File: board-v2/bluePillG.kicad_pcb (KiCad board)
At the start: 2 copper layers, 35.6 x 50.8 mm, 34 parts, among them IC1 STM32G431C6T6, J1 Conn_02x03_Odd_Even, J2 Conn_01x20_Male, J3 Conn_01x04_Male, J4 Conn_01x20_Male, U1 LM1117-3.3, Y1 32.768kHz, Y2 8MHz

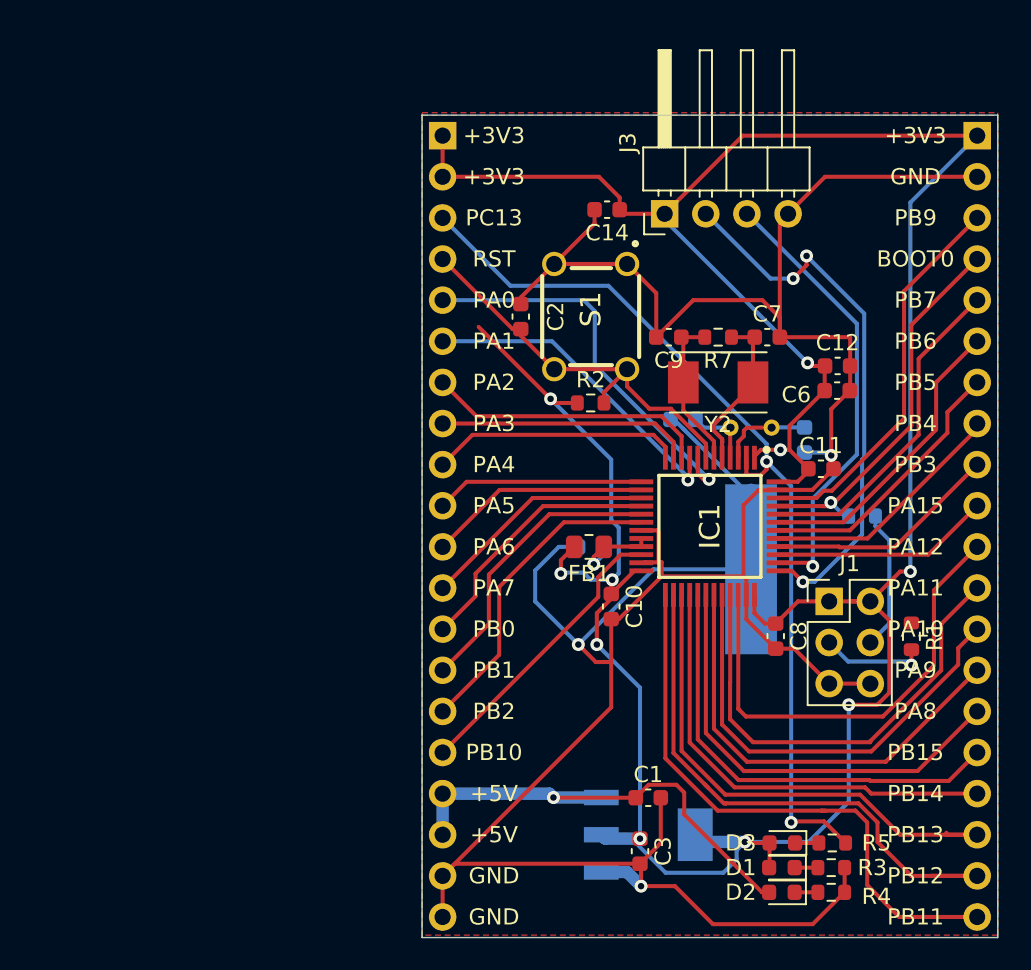
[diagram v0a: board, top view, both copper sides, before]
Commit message: board v2
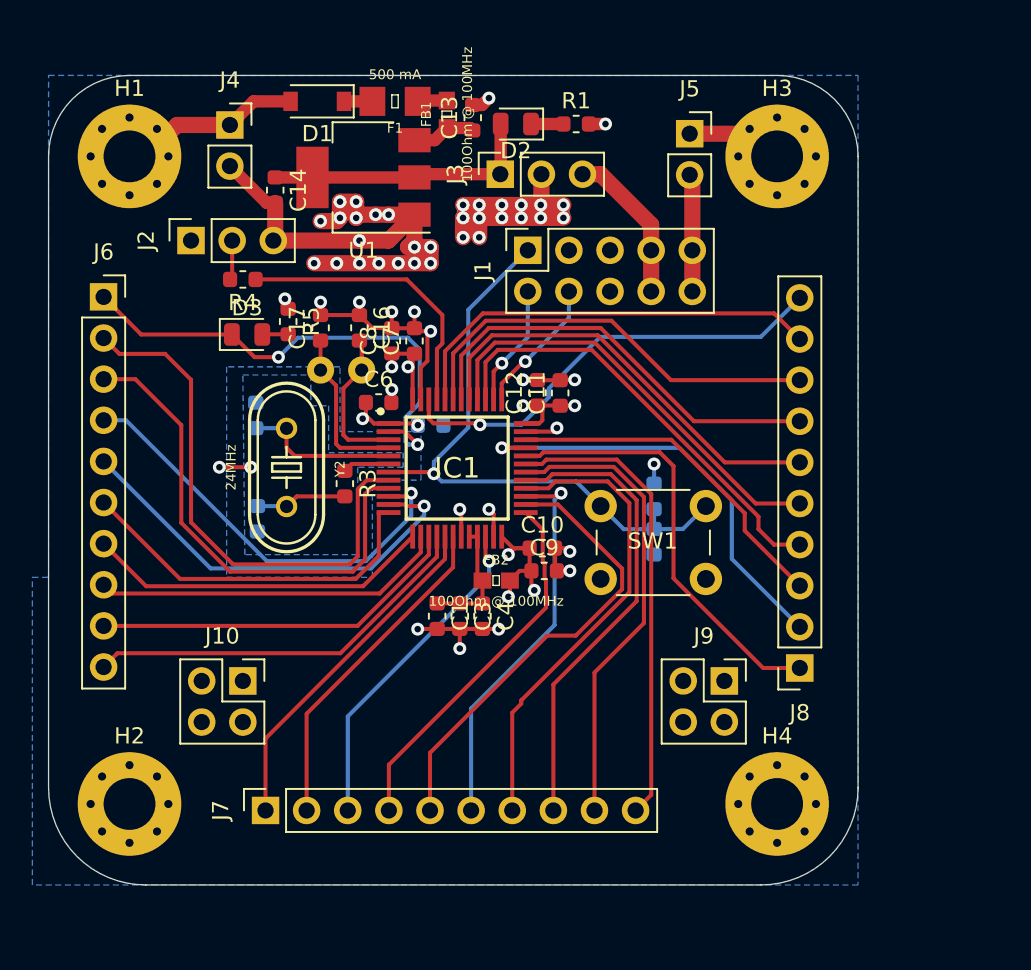
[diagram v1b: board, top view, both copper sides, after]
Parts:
- removed C2: 0.1uF, Capacitor_SMD:C_0603_1608Metric
- removed R6, R7: 100k, Resistor_SMD:R_0603_1608Metric
- removed S1: FSM4JH, FSM4JH:FSM4JH
- added C15: 100nF, Capacitor_SMD:C_0603_1608Metric, B.Cu at (66.4, 70.8)
- added C16: 6.8pF, Capacitor_SMD:C_0603_1608Metric, F.Cu at (48.2, 57.6)
- added C17: 6.8pF, Capacitor_SMD:C_0603_1608Metric, F.Cu at (45.8, 57.6)
- added C18: 20pF, Capacitor_SMD:C_0603_1608Metric, B.Cu at (41.8, 63.0)
- added C19: 20pF, Capacitor_SMD:C_0603_1608Metric, B.Cu at (41.9, 69.4)
- added F1: 500 mA, Resistors:1206, F.Cu at (50.4, 43.6)
- added FB2: 100Ohm @ 100MHz, Resistors:0603, F.Cu at (56.6, 73.2)
- added H1: MountingHole_Pad, MountingHole:MountingHole_3.2mm_M3_Pad_Via, F.Cu at (34.0, 47.0)
- added H2: MountingHole_Pad, MountingHole:MountingHole_3.2mm_M3_Pad_Via, F.Cu at (34.0, 87.0)
- added H3: MountingHole_Pad, MountingHole:MountingHole_3.2mm_M3_Pad_Via, F.Cu at (74.0, 47.0)
- added H4: MountingHole_Pad, MountingHole:MountingHole_3.2mm_M3_Pad_Via, F.Cu at (74.0, 87.0)
- added J10: Conn_02x02_Top_Bottom, Connector_PinSocket_2.54mm:PinSocket_2x02_P2.54mm_Vertical, F.Cu at (41.0, 79.4)
- added J5: Conn_01x02_Male, Connector_PinSocket_2.54mm:PinSocket_1x02_P2.54mm_Vertical, F.Cu at (68.6, 45.6)
- added J6: Conn_01x10_Male, Connector_PinSocket_2.54mm:PinSocket_1x10_P2.54mm_Vertical, F.Cu at (32.4, 55.7)
- added J7: Conn_01x10_Male, Connector_PinSocket_2.54mm:PinSocket_1x10_P2.54mm_Vertical, F.Cu at (42.4, 87.4)
- added J8: Conn_01x10_Male, Connector_PinSocket_2.54mm:PinSocket_1x10_P2.54mm_Vertical, F.Cu at (75.4, 78.6)
- added J9: Conn_02x02_Top_Bottom, Connector_PinSocket_2.54mm:PinSocket_2x02_P2.54mm_Vertical, F.Cu at (70.7, 79.4)
- added SW1: SW_Push, Button_Switch_THT:SW_PUSH_6mm_H5mm, F.Cu at (63.1, 68.6)
- C1, C3: value 0.1uF -> 1uF
- C10, C6, C8: value 0.1uF -> 100nF
- C11: value 0.1uF -> 10uF
- C12: value 10uF -> 100nF
- C13: value 0.1uF -> 10u; moved to F.Cu
- C14: value 0.1uF -> 10u
- C4: value 20p -> 100nF; moved to F.Cu
- C5, C7, C9: value 20p -> 10uF
- D1: value LED -> 1N5819; footprint LED_SMD:LED_0603_1608Metric -> Diode_SMD:D_SOD-123
- D2, D3: footprint LED_SMD:LED_0603_1608Metric -> LED_SMD:LED_0805_2012Metric
- FB1: value Ferrite_Bead -> 100Ohm @ 100MHz; footprint Resistor_SMD:R_0805_2012Metric -> Resistors:0603
- IC1: value STM32G431C6T6 -> STM32G431C6T6-STM32G431C6T6
- J1: value Conn_02x03_Odd_Even -> Conn_02x05_Odd_Even; footprint Connector_PinHeader_2.54mm:PinHeader_2x03_P2.54mm_Vertical -> Connector_PinSocket_2.54mm:PinSocket_2x05_P2.54mm_Vertical
- J2: value Conn_01x20_Male -> Conn_01x03_Male; footprint Connector_PinHeader_2.54mm:PinHeader_1x20_P2.54mm_Vertical -> Connector_PinSocket_2.54mm:PinSocket_1x03_P2.54mm_Vertical; moved to F.Cu
- J3: value Conn_01x04_Male -> Conn_01x03_Male; footprint Connector_PinHeader_2.54mm:PinHeader_1x04_P2.54mm_Horizontal -> Connector_PinSocket_2.54mm:PinSocket_1x03_P2.54mm_Vertical
- J4: value Conn_01x20_Male -> Conn_01x02_Male; footprint Connector_PinHeader_2.54mm:PinHeader_1x20_P2.54mm_Vertical -> Connector_PinSocket_2.54mm:PinSocket_1x02_P2.54mm_Vertical; moved to F.Cu
- R1: value 100k -> 2.2k
- R2: moved to B.Cu
- R3: value 1k -> 330
- R4: value 1k -> 10k
- R5: value 1k -> 2.2k
- U1: value LM1117-3.3 -> AMS1117-3.3; footprint mod:SOT-223-4 -> Package_TO_SOT_SMD:SOT-223-3_TabPin2; moved to F.Cu
- Y1: footprint Crystal:Crystal_AT310_D3.0mm_L10.0mm_Horizontal_1EP_style1 -> Clocks:CRYSTAL-PTH-2X6-CYL
- Y2: value 8MHz -> 24MHz; footprint Crystal:Crystal_SMD_Abracon_ABM7-2Pin_6.0x3.5mm -> Clocks:HC49U
- moved D1 55.4 mm to (45.6, 43.6)
- moved R4 52.5 mm to (41.0, 54.6), turned to 180 degrees
- moved D2 50.2 mm to (57.9, 45.0)
- moved R5 46.5 mm to (43.8, 57.2), turned to 270 degrees
- moved J4 46.2 mm to (40.2, 45.1), turned to 0 degrees
- moved D3 45.6 mm to (41.3, 58.0), turned to 0 degrees
- moved U1 44.2 mm to (48.5, 48.3), turned to 180 degrees
- moved R3 38.3 mm to (47.3, 67.2), turned to 270 degrees
- moved R1 37.8 mm to (61.6, 45.0), turned to 0 degrees
- moved C8 29.9 mm to (50.2, 58.4), turned to 90 degrees
- moved J1 28.6 mm to (58.6, 52.8), turned to 90 degrees
- moved C6 28.3 mm to (49.4, 62.2)
- moved FB1 28.1 mm to (53.6, 44.4), turned to 90 degrees
- moved C13 27.5 mm to (55.2, 44.6), turned to 90 degrees
- moved Y2 27.2 mm to (43.7, 66.2), turned to 270 degrees
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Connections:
- C1 pad 1: +5V -> +3.3VA
- C1 pad 2: Earth -> GND
- C10 pad 2: Earth -> GND
- C11 pad 2: Earth -> GND
- C12 pad 2: Earth -> GND
- C13 pad 1: +3.3VA -> Net-(C13-Pad1)
- C13 pad 2: Earth -> GND
- C14 pad 1: +3V3 -> +3.3VP
- C14 pad 2: Earth -> GND
- C3 pad 1: +3V3 -> +3.3VA
- C3 pad 2: Earth -> GND
- C4 pad 1: Net-(C4-Pad1) -> +3.3VA
- C4 pad 2: Earth -> GND
- C5 pad 1: Net-(C5-Pad1) -> +3V3
- C5 pad 2: Earth -> GND
- C6 pad 2: Earth -> GND
- C7 pad 1: Net-(C7-Pad1) -> +3V3
- C7 pad 2: Earth -> GND
- C8 pad 2: Earth -> GND
- C9 pad 1: Net-(C9-Pad1) -> +3V3
- C9 pad 2: Earth -> GND
- D1 pad 2: +3V3 -> VCC
- D2 pad 2: +5V -> +3.3VP
- D3 pad 1: Net-(D3-Pad1) -> PC13
- D3 pad 2: +3V3 -> Net-(D3-Pad2)
- FB1 pad 1: +3.3VA -> Net-(C13-Pad1)
- FB1 pad 2: +3V3 -> Net-(F1-Pad1)
- IC1 pad 10: /PA2 -> PA2
- IC1 pad 11: /PA3 -> PA3
- IC1 pad 12: /PA4 -> PA4
- IC1 pad 13: /PA5 -> PA5
- IC1 pad 14: /PA6 -> PA6
- IC1 pad 15: /PA7 -> PA7
- IC1 pad 16: /PB0 -> PB0
- IC1 pad 17: /PB1 -> PB1
- IC1 pad 18: /PB2 -> PB2
- IC1 pad 19: Earth -> GND
- IC1 pad 2: /PC13 -> PC13
- IC1 pad 22: /PB10 -> PB10
- IC1 pad 23: Earth -> GND
- IC1 pad 25: /PB11 -> PB11
- IC1 pad 26: /PB12 -> PB12
- IC1 pad 27: /PB13 -> PB13
- IC1 pad 28: /PB14 -> PB14
- IC1 pad 29: /PB15 -> PB15
- IC1 pad 3: Net-(C4-Pad1) -> OSC32_IN
- IC1 pad 30: /PA8 -> PA8
- IC1 pad 31: /PA9 -> PA9
- IC1 pad 32: /PA10 -> PA10
- IC1 pad 33: /PA11 -> PA11
- IC1 pad 34: /PA12 -> PA12
- IC1 pad 35: Earth -> GND
- IC1 pad 37: /SWDIO -> SWDIO
- IC1 pad 38: /SWCLK -> SWCLK
- IC1 pad 39: /PA15 -> PA15
- IC1 pad 4: Net-(C5-Pad1) -> OSC32_OUT
- IC1 pad 40: /PB3 -> PB3
- IC1 pad 41: /PB4 -> PB4
- IC1 pad 42: /PB5 -> PB5
- IC1 pad 43: /PB6 -> PB6
- IC1 pad 44: /PB7 -> PB7
- IC1 pad 45: /BOOT0 -> BOOT0
- IC1 pad 46: /PB9 -> PB9
- IC1 pad 47: Earth -> GND
- IC1 pad 5: Net-(C7-Pad1) -> OSC_IN
- IC1 pad 6: Net-(C9-Pad1) -> OSC_OUT
- IC1 pad 7: /RESET -> NRST
- IC1 pad 8: /PA0 -> PA0
- IC1 pad 9: /PA1 -> PA1
- J1 pad 1: +3V3 -> NRST
- J1 pad 2: +3V3 -> SWCLK
- J1 pad 3: Net-(J1-Pad3) -> SWIW
- J1 pad 4: Net-(J1-Pad4) -> SWDIO
- J1 pad 5: Earth -> GND
- J1 pad 6: Earth -> GND
- J2 pad 2: +3V3 -> Net-(J2-Pad2)
- J2 pad 3: /PC13 -> GND
- J3 pad 1: +3V3 -> +3.3VP
- J3 pad 2: /SWDIO -> +3V3
- J3 pad 3: /SWCLK -> +3V3S
- J4 pad 1: +3V3 -> VCC
- J4 pad 2: Earth -> GND
- R1 pad 1: /BOOT1 -> Net-(D2-Pad1)
- R1 pad 2: Net-(J1-Pad3) -> GND
- R2 pad 2: /RESET -> NRST
- R3 pad 1: Net-(D1-Pad1) -> OSC_OUT
- R3 pad 2: Earth -> Net-(C19-Pad1)
- R4 pad 1: Net-(D2-Pad1) -> BOOT0
- R4 pad 2: Earth -> Net-(J2-Pad2)
- R5 pad 1: Net-(D3-Pad1) -> +3V3
- R5 pad 2: /PC13 -> Net-(D3-Pad2)
- U1 pad 1: Earth -> GND
- U1 pad 2: +3V3 -> +3.3VP
- U1 pad 3: +5V -> Net-(C13-Pad1)
- Y1 pad 1: Net-(C4-Pad1) -> OSC32_IN
- Y1 pad 2: Net-(C5-Pad1) -> OSC32_OUT
- Y2 pad 1: Net-(C7-Pad1) -> OSC_IN
- Y2 pad 2: Net-(C9-Pad1) -> Net-(C19-Pad1)
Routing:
- net Earth: track 206.4 -> 0.00 mm, vias 3 -> 0
- net +3V3: track 196.8 -> 57.0 mm, vias 10 -> 25
- net GND: track 0.00 -> 74.2 mm, vias 0 -> 37
- net /PC13: track 56.6 -> 0.00 mm, vias 2 -> 0
- net VCC: track 0.00 -> 46.9 mm
- net NRST: track 0.00 -> 39.2 mm, vias 0 -> 1
- net /PB11: track 35.9 -> 0.00 mm
- net /PB12: track 35.5 -> 0.00 mm
- net /SWDIO: track 34.2 -> 0.00 mm, vias 3 -> 0
- net PA0: track 0.00 -> 33.1 mm
- net /PB13: track 32.1 -> 0.00 mm
- net PC13: track 0.00 -> 30.9 mm, vias 0 -> 2
- net PA1: track 0.00 -> 30.6 mm
- net +5V: track 37.2 -> 7.27 mm, vias 1 -> 0
- net /PA11: track 29.2 -> 0.00 mm
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- added copper zone on In2.Cu, net +3V3
- added copper zone on B.Cu, net GND
- added copper zone on In1.Cu, net GND
- removed copper zone on B.Cu, net Earth
- removed copper zone on F.Cu, net Earth
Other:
- board size 35.6 x 50.8 mm -> 50 x 50 mm
- copper layers 2 -> 4
- board text removed: "+3V3"
- board text removed: "+5V"
- board text removed: "BOOT0"
- board text removed: "GND"
- board text removed: "PA0"
- board text removed: "PA1"
- board text removed: "PA10"
- board text removed: "PA11"
- board text removed: "PA12"
- board text removed: "PA15"
- board text removed: "PA2"
- board text removed: "PA3"
- board text removed: "PA4"
- board text removed: "PA5"
- board text removed: "PA6"
- board text removed: "PA7"
- board text removed: "PA8"
- board text removed: "PA9"
- board text removed: "PB0"
- board text removed: "PB1"
- board text removed: "PB10"
- board text removed: "PB11"
- board text removed: "PB12"
- board text removed: "PB13"
- board text removed: "PB14"
- board text removed: "PB15"
- board text removed: "PB2"
- board text removed: "PB3"
- board text removed: "PB4"
- board text removed: "PB5"
- board text removed: "PB6"
- board text removed: "PB7"
- board text removed: "PB9"
- board text removed: "PC13"
- board text removed: "RST"
